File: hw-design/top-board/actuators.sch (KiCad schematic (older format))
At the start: 39 parts, among them J1 Conn_01x10_Male, SW2 JB15HBPC-JB, SW3 JB15HBPC-JB, SW4 JB15HBPC-JB, SW5 JB15HBPC-JB, SW6 JB15HBPC-JB, SW7 JB15HBPC-JB, SW8 JB15HBPC-JB, U6 74HC4051

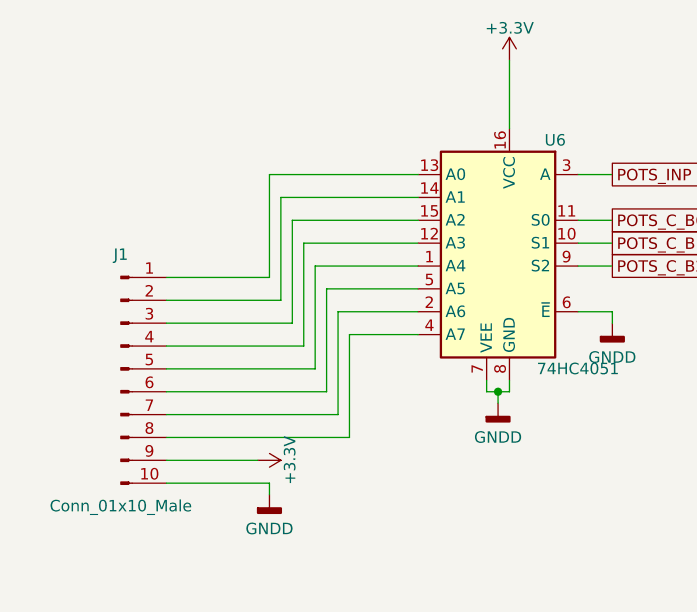
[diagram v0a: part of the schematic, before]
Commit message: routing tracks
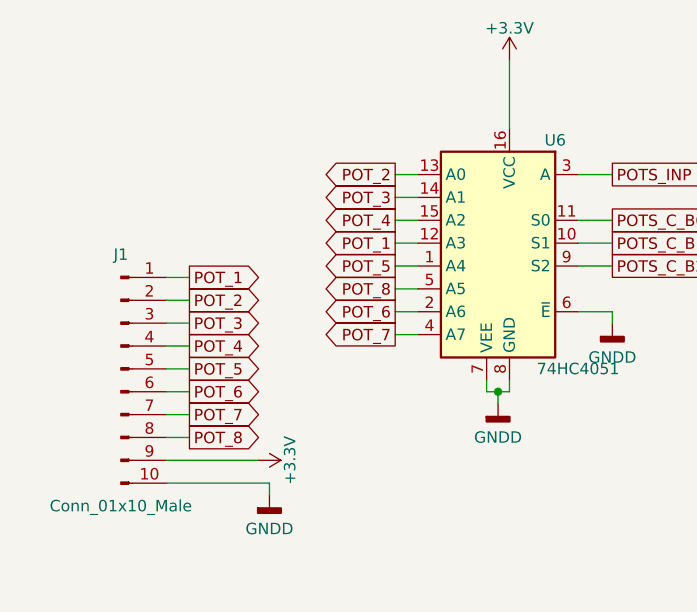
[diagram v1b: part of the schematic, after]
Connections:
- net labels added: POT_1, POT_2, POT_3, POT_4, POT_5, POT_6, POT_7, POT_8
- wire segments 137 -> 129
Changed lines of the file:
@@
 Text GLabel 1250 3950 2    50   Output ~ 0
 LED_SYS_B1
+$Comp
+L +3.3V #PWR098
+U 1 1 5AF2313E
+P 2450 6500
+F 0 "#PWR098" H 2450 6350 50  0001 C CNN
+F 1 "+3.3V" H 2450 6640 50  0000 C CNN
+F 2 "" H 2450 6500 60  0000 C CNN
+F 3 "" H 2450 6500 60  0000 C CNN
+	1    2450 6500
+	-1   0    0    1
+$EndComp
+Text GLabel 2100 1450 0    50   Output ~ 0
+POT_2
+Text GLabel 2100 1550 0    50   Output ~ 0
+POT_3
+Text GLabel 2100 1650 0    50   Output ~ 0
+POT_4
+Text GLabel 2100 1750 0    50   Output ~ 0
+POT_1
+Text GLabel 2100 1850 0    50   Output ~ 0
+POT_5
+Text GLabel 2100 1950 0    50   Output ~ 0
+POT_8
+Text GLabel 2100 2050 0    50   Output ~ 0
+POT_6
+Text GLabel 2100 2150 0    50   Output ~ 0
+POT_7
+Text GLabel 1200 2600 2    50   Output ~ 0
+POT_8
+Text GLabel 1200 2500 2    50   Output ~ 0
+POT_7
+Text GLabel 1200 2400 2    50   Output ~ 0
+POT_6
+Text GLabel 1200 2300 2    50   Output ~ 0
+POT_5
+Text GLabel 1200 2200 2    50   Output ~ 0
+POT_4
+Text GLabel 1200 2100 2    50   Output ~ 0
+POT_3
+Text GLabel 1200 2000 2    50   Output ~ 0
+POT_2
+Text GLabel 1200 1900 2    50   Output ~ 0
+POT_1
 Wire Wire Line
 	10150 5450 10600 5450
@@
 	1100 2700 1500 2700
 Wire Wire Line
-	1100 1900 1550 1900
-Wire Wire Line
-	1100 2000 1600 2000
-Wire Wire Line
-	1100 2100 1650 2100
-Wire Wire Line
-	1100 2200 1700 2200
-Wire Wire Line
-	1100 2300 1750 2300
-Wire Wire Line
-	1100 2400 1800 2400
-Wire Wire Line
-	1100 2500 1850 2500
-Wire Wire Line
-	1100 2600 1900 2600
-Wire Wire Line
 	2500 2400 2600 2400
 Wire Wire Line
@@
 	2600 950  2600 1250
 Wire Wire Line
-	1550 1450 2200 1450
-Wire Wire Line
-	1600 1550 2200 1550
-Wire Wire Line
-	1650 1650 2200 1650
-Wire Wire Line
-	1700 1750 2200 1750
-Wire Wire Line
-	1750 1850 2200 1850
-Wire Wire Line
-	1800 1950 2200 1950
-Wire Wire Line
-	1850 2050 2200 2050
-Wire Wire Line
-	1900 2150 2200 2150
-Wire Wire Line
 	3050 2100 3050 2050
 Wire Wire Line
@@
 	1150 3950 1150 4000
 Wire Wire Line
-	1900 2600 1900 2150
-Wire Wire Line
-	1850 2500 1850 2050
-Wire Wire Line
-	1800 2400 1800 1950
-Wire Wire Line
-	1750 2300 1750 1850
-Wire Wire Line
-	1700 2200 1700 1750
-Wire Wire Line
-	1650 2100 1650 1650
-Wire Wire Line
-	1600 2000 1600 1550
-Wire Wire Line
-	1550 1900 1550 1450
-Wire Wire Line
 	8250 3000 8300 3000
 Wire Wire Line
@@
 Wire Wire Line
 	2850 6100 2750 6100
-$Comp
-L +3.3V #PWR098
-U 1 1 5AF2313E
-P 2450 6500
-F 0 "#PWR098" H 2450 6350 50  0001 C CNN
-F 1 "+3.3V" H 2450 6640 50  0000 C CNN
-F 2 "" H 2450 6500 60  0000 C CNN
-F 3 "" H 2450 6500 60  0000 C CNN
-	1    2450 6500
-	-1   0    0    1
-$EndComp
 Wire Wire Line
 	2450 6400 2450 6500
@@
 Wire Wire Line
 	4900 5550 4700 5550
+Wire Wire Line
+	2200 1650 2100 1650
+Wire Wire Line
+	2200 1750 2100 1750
+Wire Wire Line
+	2200 1850 2100 1850
+Wire Wire Line
+	2200 1950 2100 1950
+Wire Wire Line
+	2200 2050 2100 2050
+Wire Wire Line
+	2200 2150 2100 2150
+Wire Wire Line
+	1200 1900 1100 1900
+Wire Wire Line
+	1200 2100 1100 2100
+Wire Wire Line
+	1200 2200 1100 2200
+Wire Wire Line
+	1200 2300 1100 2300
+Wire Wire Line
+	1200 2400 1100 2400
+Wire Wire Line
+	1200 2500 1100 2500
+Wire Wire Line
+	1200 2600 1100 2600
+Wire Wire Line
+	2100 1550 2200 1550
+Wire Wire Line
+	2100 1450 2200 1450
+Wire Wire Line
+	1100 2000 1200 2000
 $EndSCHEMATC
